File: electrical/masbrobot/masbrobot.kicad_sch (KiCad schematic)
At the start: 30 parts

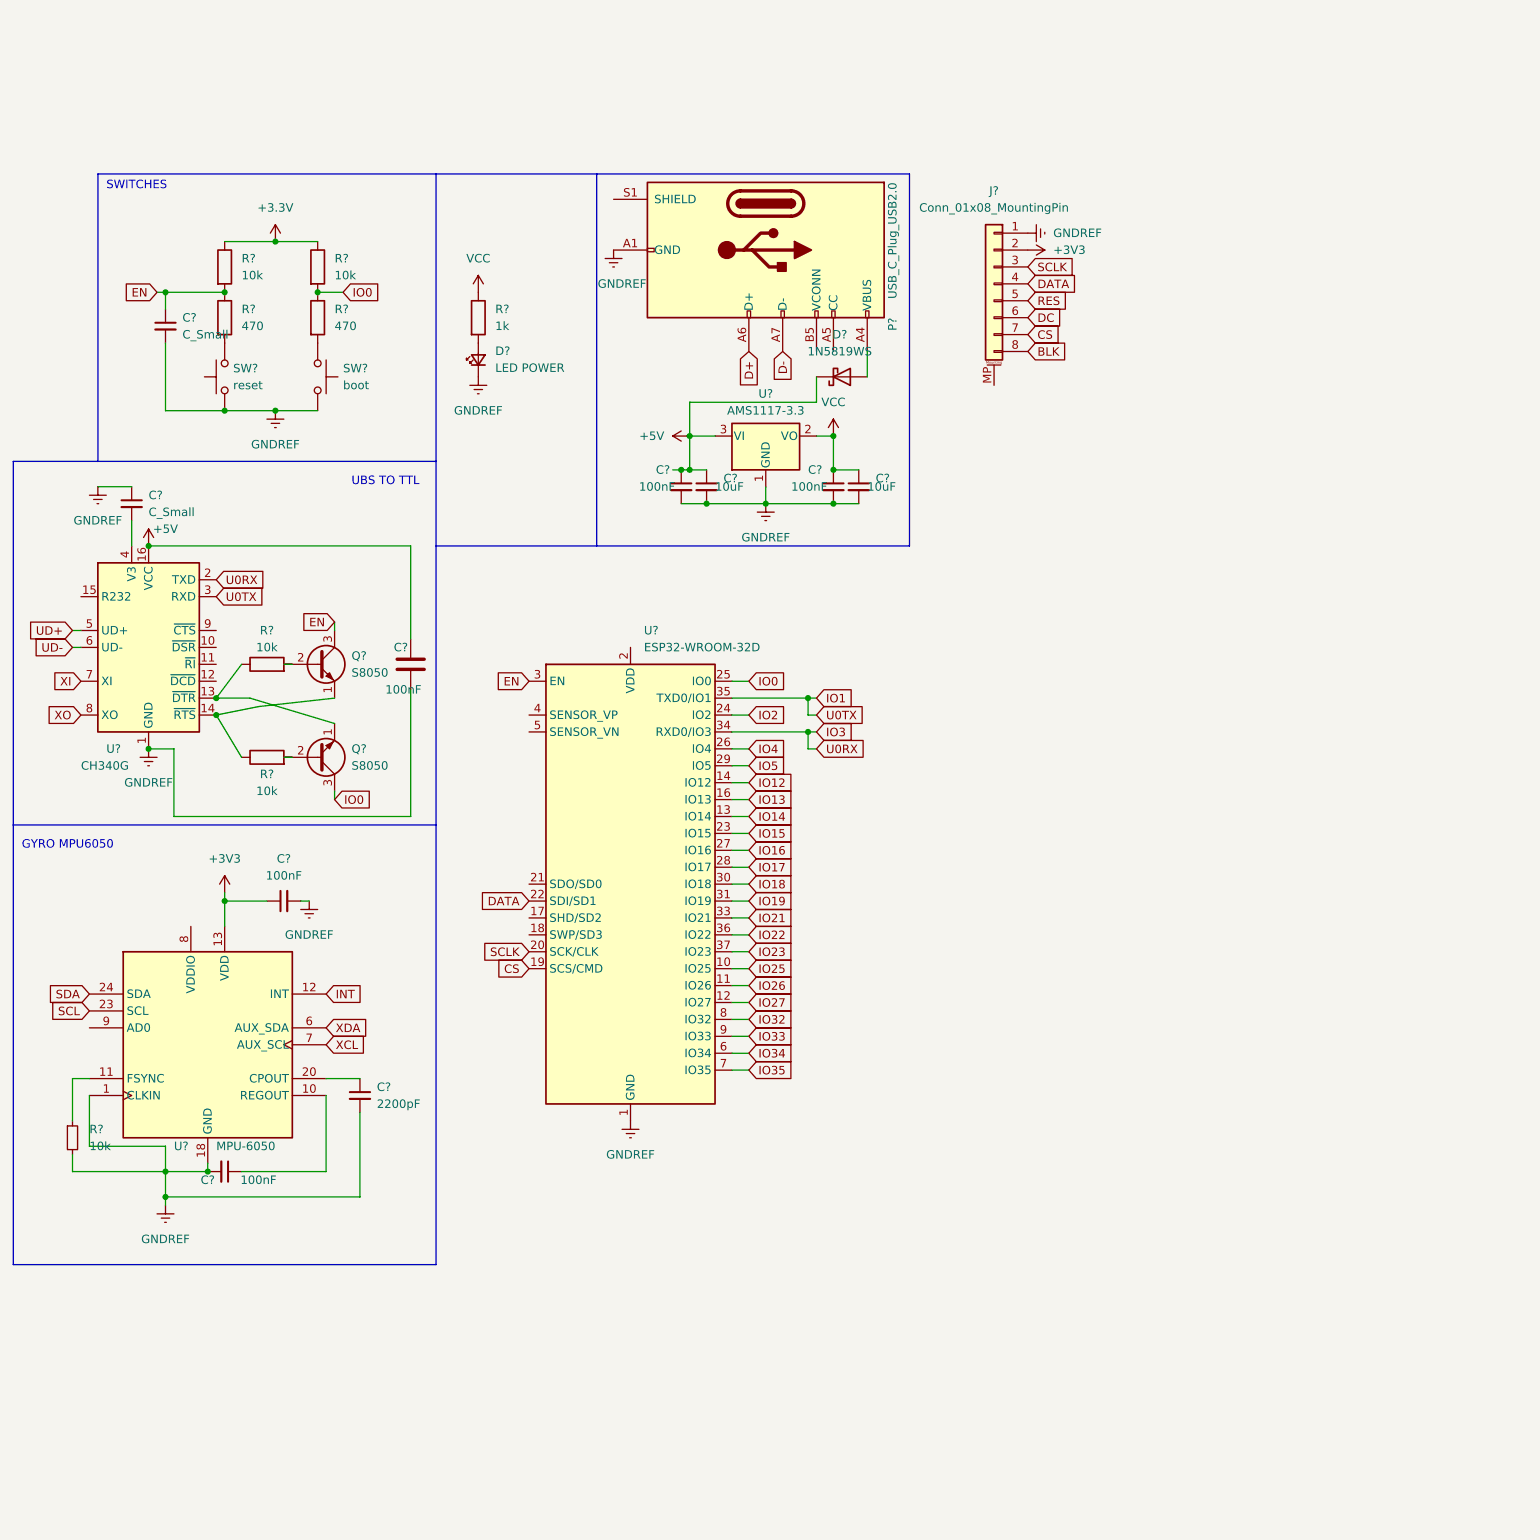
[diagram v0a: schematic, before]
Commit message: update schematic and PCB board
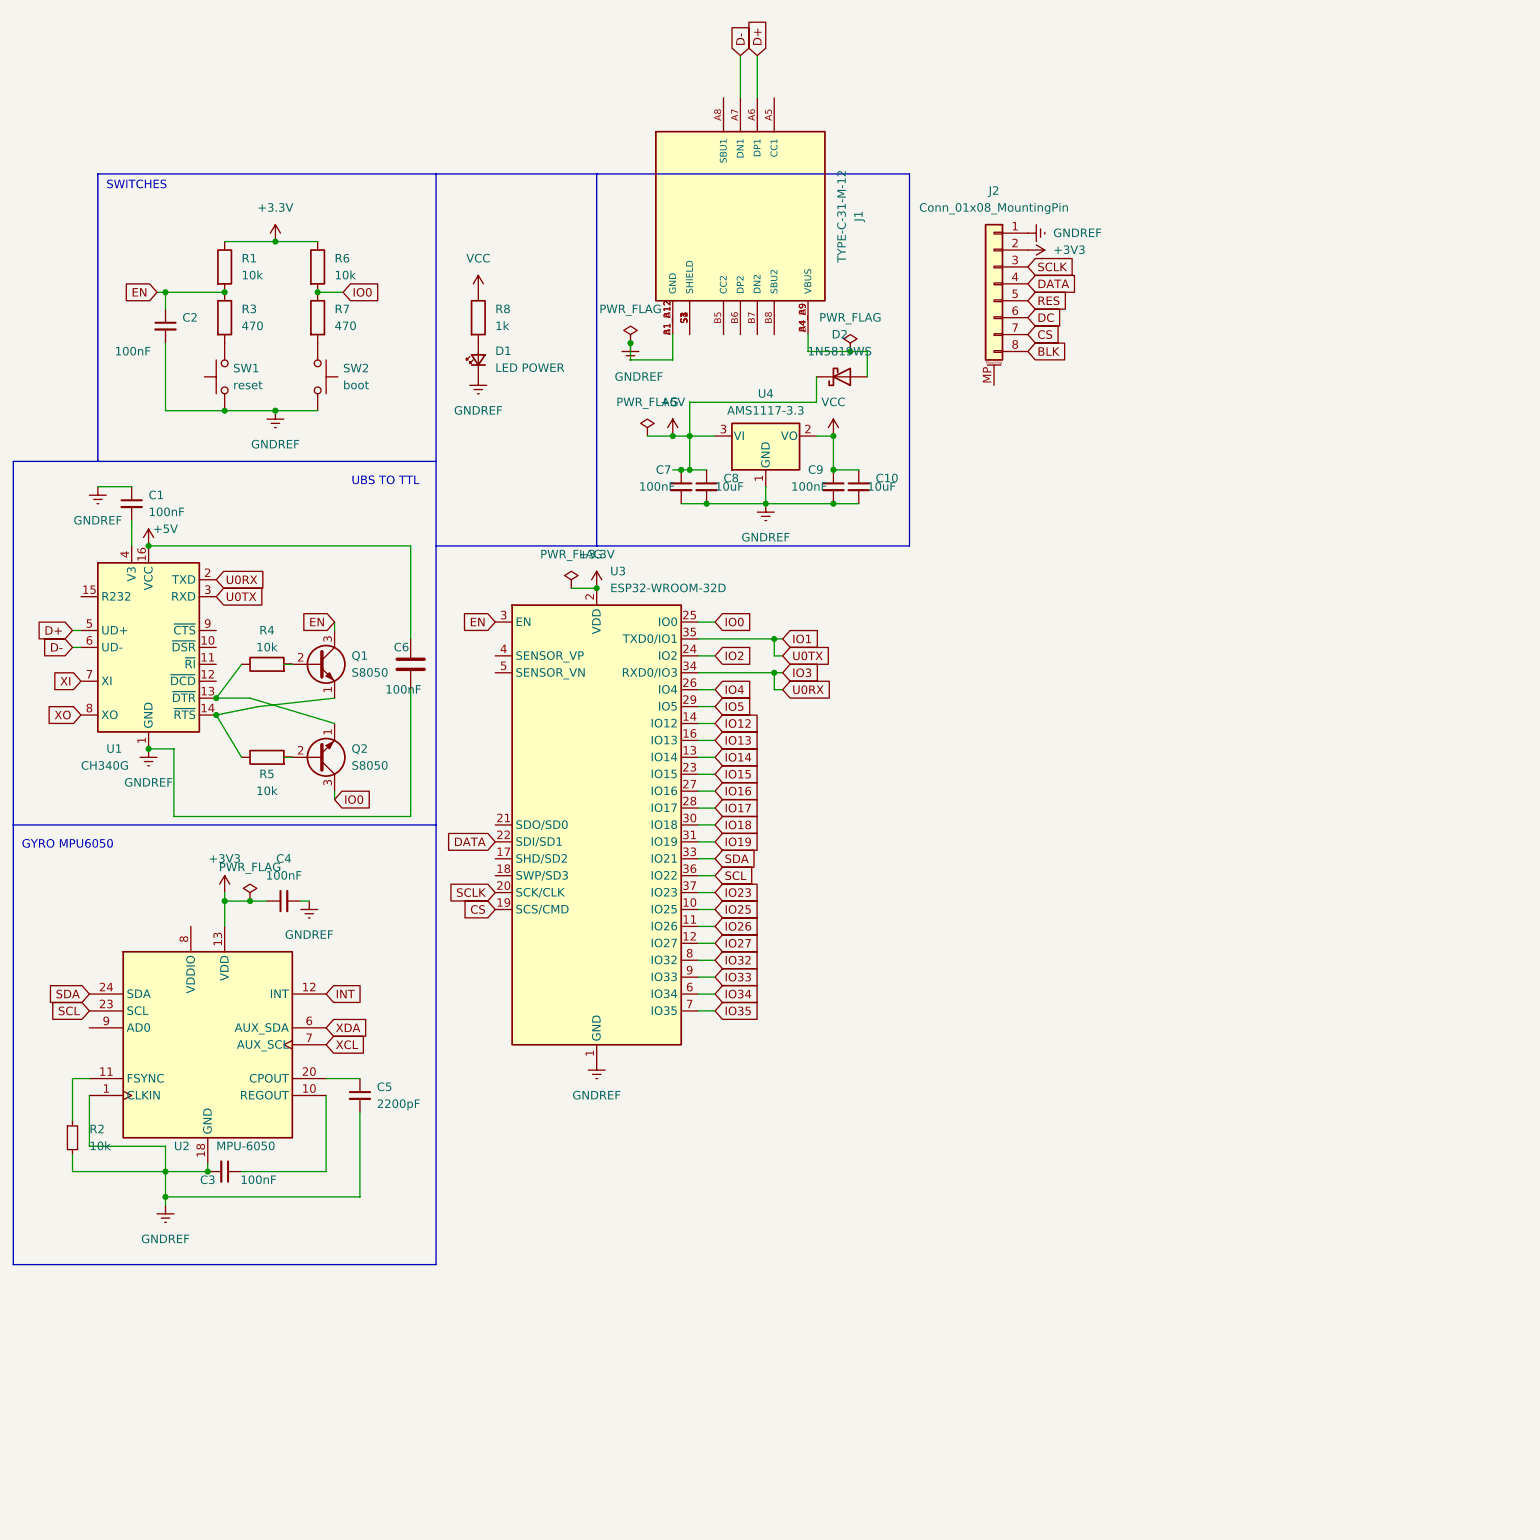
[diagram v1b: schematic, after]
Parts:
- removed P?: USB_C_Plug_USB2.0, symbol Connector:USB_C_Plug_USB2.0
- added J1: TYPE-C-31-M-12, HRO_TYPE-C-31-M-12, symbol TYPE-C-31-M-12:TYPE-C-31-M-12
- C1, C2: renamed from C?; value C_Small -> 100nF
- C10, C8: renamed from C?; footprint (none) -> Capacitor_SMD:C_0201_0603Metric
- C7, C9: renamed from C?; footprint (none) -> Capacitor_SMD:C_0805_2012Metric
- D1: renamed from D?; footprint (none) -> LED_SMD:LED_0201_0603Metric
- J2: renamed from J?; footprint (none) -> Connector_PinHeader_1.00mm:PinHeader_1x08_P1.00mm_Horizontal
- R1, R3, R6, R7: renamed from R?; footprint (none) -> Resistor_SMD:R_1206_3216Metric
- R8: renamed from R?; footprint (none) -> Resistor_SMD:R_0201_0603Metric
- SW1, SW2: renamed from SW?; footprint (none) -> Button_Switch_SMD:SW_Tactile_SPST_NO_Straight_CK_PTS636Sx25SMTRLFS
- gave numbers to parts that had none: 14
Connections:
- net IO21 is gone; now on net SDA: U3.33 (IO21)
- net IO22 is gone; now on net SCL: U3.36 (IO22)
- net UD+ is gone; now on net D+: U1.5 (UD+)
- net UD- is gone; now on net D-: U1.6 (UD-)
- net +3.3V: now also U3.2 (VDD)
- net D+: now also J1.A6 (DP1)
- net D-: now also J1.A7 (DN1)
- net GNDREF: now also J1.A1_B12 (GND), J1.B1_A12 (GND)
- net at D2.2 (A): now also J1.A4_B9 (VBUS), J1.B4_A9 (VBUS)
- new net: J1.S1 (SHIELD), J1.S2 (SHIELD), J1.S3 (SHIELD), J1.S4 (SHIELD)
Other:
- moved on the sheet: U3

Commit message: update electrial FIX.
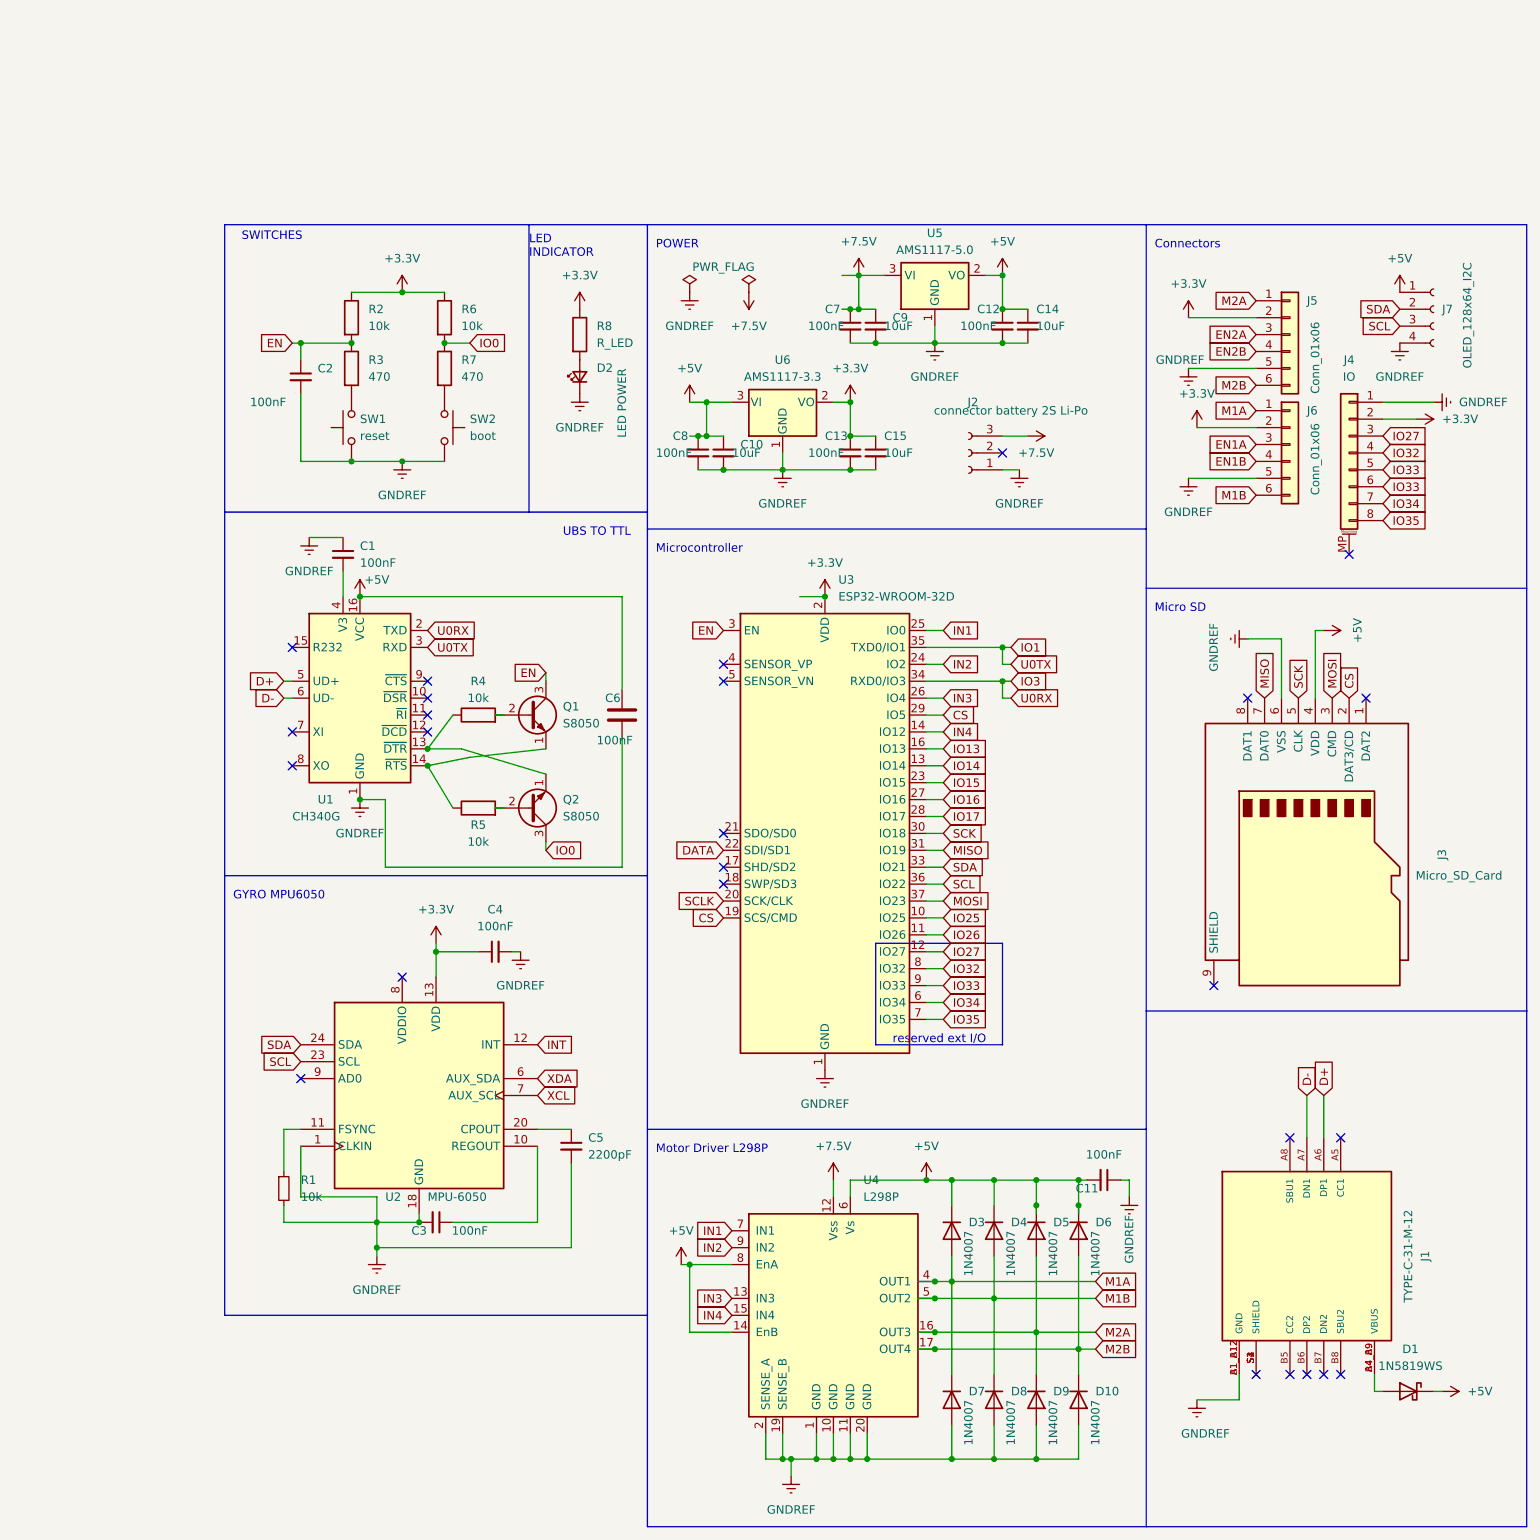
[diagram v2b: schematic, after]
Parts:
- added C11, C12, C7: 100nF, Capacitor_SMD:C_0805_2012Metric, symbol Device:C_Small
- added C14, C9: 10uF, Capacitor_SMD:C_0201_0603Metric, symbol Device:C_Small
- added D10, D3, D4, D5, D6, D7, D8, D9: 1N4007, Diode_SMD:D_0201_0603Metric, symbol Diode:1N4007
- added J2: connector battery 2S Li-Po, Connector_JST:JST_XH_S3B-XH-A-1_1x03_P2.50mm_Horizontal, symbol Connector:Conn_01x03_Socket
- added J3: Micro_SD_Card, Connector_Card:microSD_HC_Hirose_DM3BT-DSF-PEJS, symbol Connector:Micro_SD_Card
- added J5, J6: Conn_01x06, Connector_JST:JST_GH_BM06B-GHS-TBT_1x06-1MP_P1.25mm_Vertical, symbol Connector_Generic:Conn_01x06
- added J7: OLED_128x64_I2C, Connector_JST:JST_GH_BM04B-GHS-TBT_1x04-1MP_P1.25mm_Vertical, symbol Connector:Conn_01x04_Socket
- added U4: L298P, L298P:SOIC127P1420X360-20N, symbol Driver_Motor:L298P
- added U5: AMS1117-5.0, Package_TO_SOT_SMD:SOT-223-3_TabPin2, symbol Regulator_Linear:AMS1117-5.0
- C1, C2, C3, C4, C5, C6: footprint (none) -> Capacitor_SMD:C_0805_2012Metric
- D2: renamed from D1; footprint LED_SMD:LED_0201_0603Metric -> LED_SMD:LED_1206_3216Metric
- J1: footprint HRO_TYPE-C-31-M-12 -> TYPE-C-31-M-12:HRO_TYPE-C-31-M-12
- J4: renamed from J2; value Conn_01x08_MountingPin -> IO; footprint Connector_PinHeader_1.00mm:PinHeader_1x08_P1.00mm_Horizontal -> Connector_PinHeader_1.27mm:PinHeader_1x08_P1.27mm_Horizontal
- R1: renamed from R2; footprint (none) -> Resistor_SMD:R_0805_2012Metric
- R4, R5: footprint (none) -> Resistor_SMD:R_0805_2012Metric
- R8: value 1k -> R_LED; footprint Resistor_SMD:R_0201_0603Metric -> Resistor_SMD:R_0402_1005Metric
- renumbered C8 to C10, C9 to C13, C10 to C15, C7 to C8, D2 to D1, R1 to R2, U4 to U6
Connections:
- net +3V3 is gone; now on net +3.3V: C4.1, J4.2 (Pin_2), U2.13 (VDD)
- net BLK is gone; now on net IO35: J4.8 (Pin_8)
- net DC is gone; now on net IO33: J4.6 (Pin_6)
- net IO5 is gone; now on net CS: U3.29 (IO5)
- net RES is gone; now on net IO33: J4.5 (Pin_5)
- net VCC is gone; now on net +3.3V: C13.1, C15.1, R8.1, U6.2 (VO)
- net +3.3V: now also J5.2 (Pin_2), J6.2 (Pin_2)
- net +5V: now also C11.2, C12.1, C14.1, D3.1 (K), D4.1 (K), D5.1 (K), D6.1 (K), J3.4 (VDD), J7.1 (Pin_1), U4.14 (EnB), U4.6 (Vs), U4.8 (EnA), U5.2 (VO)
- net CS: now also J3.2 (DAT3/CD); no longer J4.7 (Pin_7)
- net DATA: no longer J4.4 (Pin_4)
- net GNDREF: now also C11.1, C12.2, C14.2, C7.2, C9.2, D10.2 (A), D7.2 (A), D8.2 (A), D9.2 (A), J2.1 (Pin_1), J3.6 (VSS), J5.5 (Pin_5), J6.5 (Pin_5), J7.4 (Pin_4), U4.1 (GND), U4.10 (GND), U4.11 (GND), U4.19 (SENSE_B), U4.2 (SENSE_A), U4.20 (GND), U5.1 (GND)
- net IO0: no longer U3.25 (IO0)
- net IO27: now also J4.3 (Pin_3)
- net IO32: now also J4.4 (Pin_4)
- net IO34: now also J4.7 (Pin_7)
- net SCL: now also J7.3 (Pin_3)
- net SCLK: no longer J4.3 (Pin_3)
- net SDA: now also J7.2 (Pin_2)
- net IO12 renamed IN4
- net IN4: now also U4.15 (IN4)
- net IO18 renamed SCK
- net SCK: now also J3.5 (CLK)
- net IO19 renamed MISO
- net MISO: now also J3.7 (DAT0)
- net IO2 renamed IN2
- net IN2: now also U4.9 (IN2)
- net IO23 renamed MOSI
- net MOSI: now also J3.3 (CMD)
- net IO4 renamed IN3
- net IN3: now also U4.13 (IN3)
- net XI: no longer names the net of U1.7 (XI)
- net XO: no longer names the net of U1.8 (XO)
- new net +7.5V: C7.1, C9.1, J2.3 (Pin_3), U4.12 (Vss), U5.3 (VI)
- new net EN1A: J6.3 (Pin_3)
- new net EN1B: J6.4 (Pin_4)
- new net EN2A: J5.3 (Pin_3)
- new net EN2B: J5.4 (Pin_4)
- new net IN1: U3.25 (IO0), U4.7 (IN1)
- new net M1A: D3.2 (A), D7.1 (K), J6.1 (Pin_1), U4.4 (OUT1)
- new net M1B: D4.2 (A), D8.1 (K), J6.6 (Pin_6), U4.5 (OUT2)
- new net M2A: D5.2 (A), D9.1 (K), J5.1 (Pin_1), U4.16 (OUT3)
- new net M2B: D10.1 (K), D6.2 (A), J5.6 (Pin_6), U4.17 (OUT4)
- no-connect marks 0 -> 26
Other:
- note added: "Connectors"
- note added: "LED INDICATOR"
- note added: "Micro SD"
- note added: "Microcontroller"
- note added: "Motor Driver L298P"
- note added: "POWER"
- note added: "reserved ext I/O"
- company: (none) -> TRKB/FTMM/Universitas Airlangga
- title: (none) -> Schematic Masbrobot, PCB 1
- moved on the sheet: C1, C10, C13, C15, C2, C3, C4, C5, C6, C8, D1, D2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
